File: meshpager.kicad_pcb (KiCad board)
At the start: 4 copper layers, 82.5 x 90 mm, 105 parts, among them J1 Conn_01x05, J2 Conn_01x03, J3 009155003301006, J4 USB_C_Receptacle_USB2.0_16P, J5 S8B-PH-SM4-TB, J6 HC-FPC-05-09-5RLTAG, J7 HC-FPC-05-09-5RLTAG, Q1 NCE40P05Y, SW1 SW_SPST, SW2 MK-12C02-G020, U1 RAK4630-8-SM-I, U2 SGM2578AADYG/TR, U3 SY6287CABC, U4 SGM6036-3.3YUDT6G/TR, U5 SGM41524YTDC8G/TR, U6 USBLC6-2SC6, U7 TCA8418RTWR

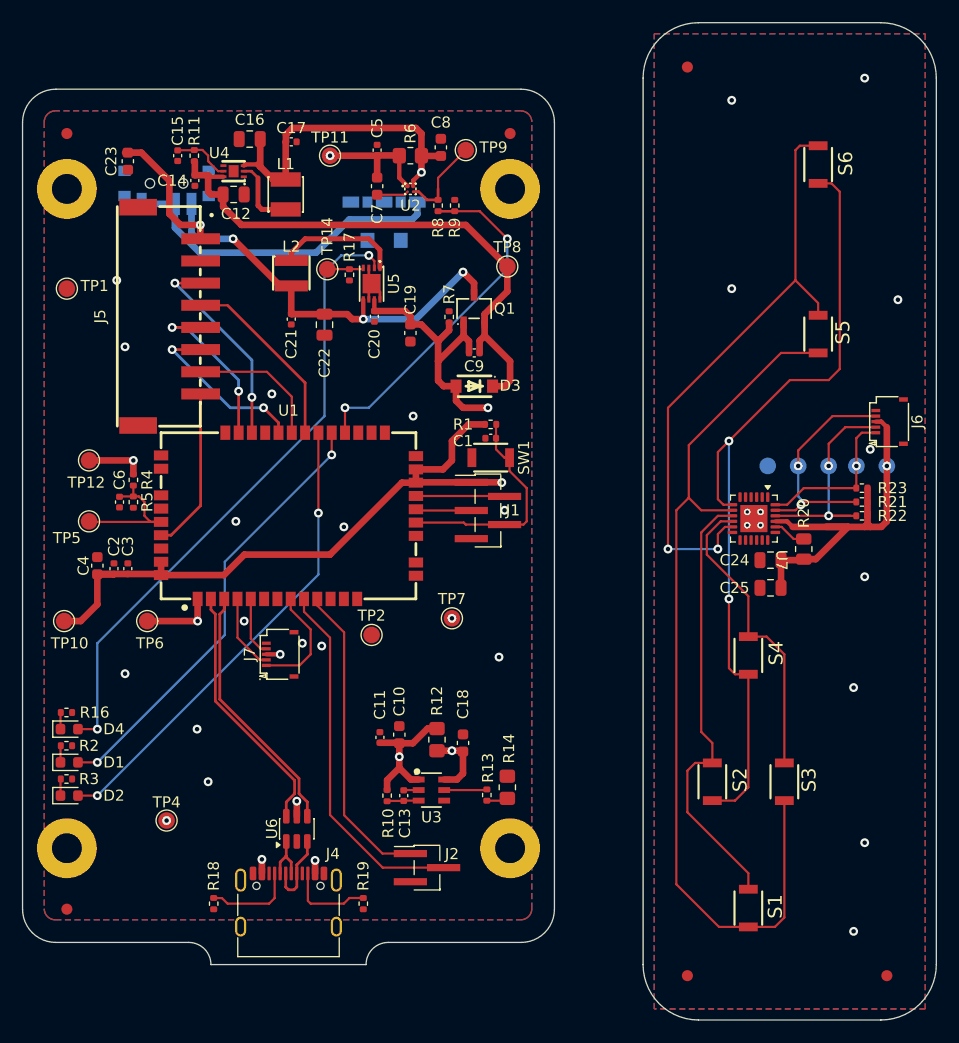
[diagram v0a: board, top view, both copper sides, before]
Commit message: Update
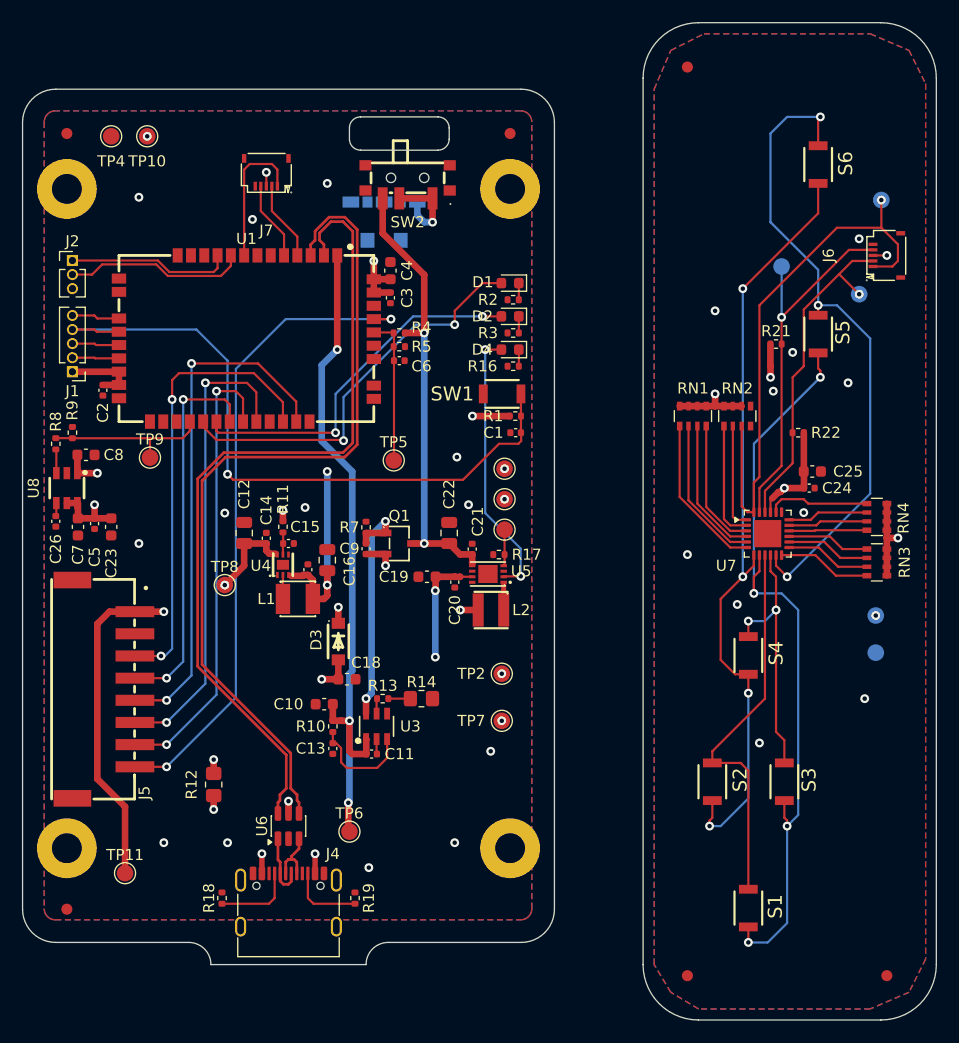
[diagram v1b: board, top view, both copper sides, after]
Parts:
- removed R20: 10K, Resistor_SMD:R_0805_2012Metric
- removed R23: 10K, Resistor_SMD:R_0402_1005Metric
- removed R6: 0, Resistor_SMD:R_0805_2012Metric_Pad1.20x1.40mm_HandSolder
- removed U2: SGM2578AADYG/TR, pager-jlc:WLCSP-4_L0.9-W0.9-R2-C2-P0.50-TL
- added C26: 1nF, Capacitor_SMD:C_0402_1005Metric, F.Cu at (103.0, 89.0)
- added RN1: R_Pack04, Resistor_SMD:R_Array_Convex_4x0603, F.Cu at (160.5, 79.5)
- added RN2: R_Pack04, Resistor_SMD:R_Array_Convex_4x0603, F.Cu at (164.5, 79.5)
- added RN3: R_Pack04, Resistor_SMD:R_Array_Convex_4x0603, F.Cu at (177.1, 92.7)
- added RN4: R_Pack04, Resistor_SMD:R_Array_Convex_4x0603, F.Cu at (177.1, 88.6)
- added U8: TPS22918DBVR, pager-jlc:SOT-23-6_L2.9-W1.6-P0.95-LS2.8-BR, F.Cu at (104.0, 86.0)
- C24: footprint Capacitor_SMD:C_0805_2012Metric -> Capacitor_SMD:C_0402_1005Metric
- C25: footprint Capacitor_SMD:C_0805_2012Metric -> Capacitor_SMD:C_0603_1608Metric
- D1: value LED -> GREEN
- D2: value LED -> BLUE
- J1: footprint Connector_PinHeader_1.27mm:PinHeader_1x05_P1.27mm_Vertical_SMD_Pin1Left -> Connector_PinHeader_1.27mm:PinHeader_1x05_P1.27mm_Vertical
- J2: footprint Connector_PinHeader_1.27mm:PinHeader_1x03_P1.27mm_Vertical_SMD_Pin1Left -> Connector_PinHeader_1.27mm:PinHeader_1x03_P1.27mm_Vertical
- R13: value 470 1% -> 470
- SW1: value SW_SPST -> B3U-1000P
- SW2: moved to F.Cu
- moved TP11 67.3 mm to (109.2, 120.8)
- moved J2 63.5 mm to (104.5, 65.5)
- moved TP4 62.0 mm to (108.0, 54.2)
- moved D1 58.8 mm to (144.0, 67.5), turned to 180 degrees
- moved D2 58.8 mm to (144.0, 70.5), turned to 180 degrees
- moved R2 57.0 mm to (144.3, 69.0), turned to 180 degrees
- moved R3 57.0 mm to (144.3, 72.0), turned to 180 degrees
- moved D4 52.5 mm to (144.0, 73.5), turned to 180 degrees
- moved R16 51.0 mm to (144.3, 75.0), turned to 0 degrees
- moved TP10 44.4 mm to (111.2, 54.2)
- moved J7 43.5 mm to (122.0, 57.5), turned to 180 degrees
- moved TP1 42.7 mm to (143.5, 84.2)
- moved C8 42.4 mm to (105.7, 83.0), turned to 0 degrees
- moved C5 42.3 mm to (106.5, 89.2), turned to -90 degrees
- moved C7 40.9 mm to (105.0, 89.5)
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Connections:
- net /input_module/TCA_KEYPAD_INT renamed /input_module/INT
- J7 pad 3: +3V3_S -> +3V3
- R8 pad 1: /mcu/IO2 -> Net-(U8-ON)
- R8 pad 2: Net-(U2-ON) -> /mcu/IO2
- TP9 pad 1: Net-(U2-ON) -> /mcu/IO2
- U7 pad 1: unconnected-(U7-ROW7-Pad1) -> Net-(RN2-R2.1)
- U7 pad 12: unconnected-(U7-COL3-Pad12) -> Net-(RN3-R1.2)
- U7 pad 13: unconnected-(U7-COL4-Pad13) -> Net-(RN3-R2.2)
- U7 pad 14: unconnected-(U7-COL5-Pad14) -> Net-(RN3-R3.2)
- U7 pad 15: unconnected-(U7-COL6-Pad15) -> Net-(RN3-R4.2)
- U7 pad 16: unconnected-(U7-COL7-Pad16) -> Net-(RN4-R1.2)
- U7 pad 17: unconnected-(U7-COL8-Pad17) -> Net-(RN4-R2.2)
- U7 pad 18: unconnected-(U7-COL9-Pad18) -> Net-(RN4-R3.2)
- U7 pad 2: unconnected-(U7-ROW6-Pad2) -> Net-(RN2-R1.1)
- U7 pad 3: unconnected-(U7-ROW5-Pad3) -> Net-(RN1-R4.1)
- U7 pad 4: unconnected-(U7-ROW4-Pad4) -> Net-(RN1-R3.1)
- U7 pad 5: unconnected-(U7-ROW3-Pad5) -> Net-(RN1-R2.1)
- U7 pad 6: unconnected-(U7-ROW2-Pad6) -> Net-(RN1-R1.1)
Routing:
- net +3V3: track 120.4 -> 38.4 mm, vias 2 -> 7
- net VDD: track 35.8 -> 97.2 mm, vias 1 -> 6
- net +3V3_S: track 97.9 -> 36.6 mm, vias 3 -> 2
- net /mcu/USB_P: track 23.1 -> 75.6 mm
- net /mcu/USB_N: track 23.1 -> 74.2 mm
- net /edp/EPD.BUSY: track 14.8 -> 58.6 mm, vias 0 -> 2
- net /mcu/NRF_RESET: track 20.3 -> 62.1 mm, vias 0 -> 1
- net +BATT: track 82.8 -> 41.9 mm
- net VDC: track 51.4 -> 13.3 mm, vias 0 -> 4
- net /input_module/INT: track 14.4 -> 49.9 mm
- net Net-(D4-A): track 57.4 -> 24.8 mm
- net /edp/EPD.CS: track 15.3 -> 46.7 mm
- net /edp/EPD.RST: track 12.4 -> 41.2 mm, vias 0 -> 2
- net +5V: track 65.0 -> 36.9 mm, vias 3 -> 7
- net /edp/EPD.DC: track 15.8 -> 42.4 mm
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- added copper zone on In2.Cu, net +3V3
- added copper zone on In2.Cu, net +3V3_S
- added copper zone on In2.Cu, net +5V
- added copper zone on In2.Cu, net +BATT
- added copper zone on In2.Cu, net VBUS
- added copper zone on In2.Cu, net VDC
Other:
- outline, holes or cut-outs redrawn
- board text added: "3V3"
- board text added: "3V3S"
- board text added: "5V"
- board text added: "BATT"
- board text added: "CELL"
- board text added: "VBUS"
- board text added: "VDC"
